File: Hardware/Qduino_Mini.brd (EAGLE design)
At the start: 38.1 x 25.4 mm, 45 parts, among them Q1 PFET, U1 ATMEGA32U41:1-LESS_PASTE, U2 MCP73831, U3 MAX17048, U4 TPS78233, U5 MIGHTYQ-L-SILK, U6 MIGHTYQ-S-SILK, U7 DNP, Y1 8MHZ

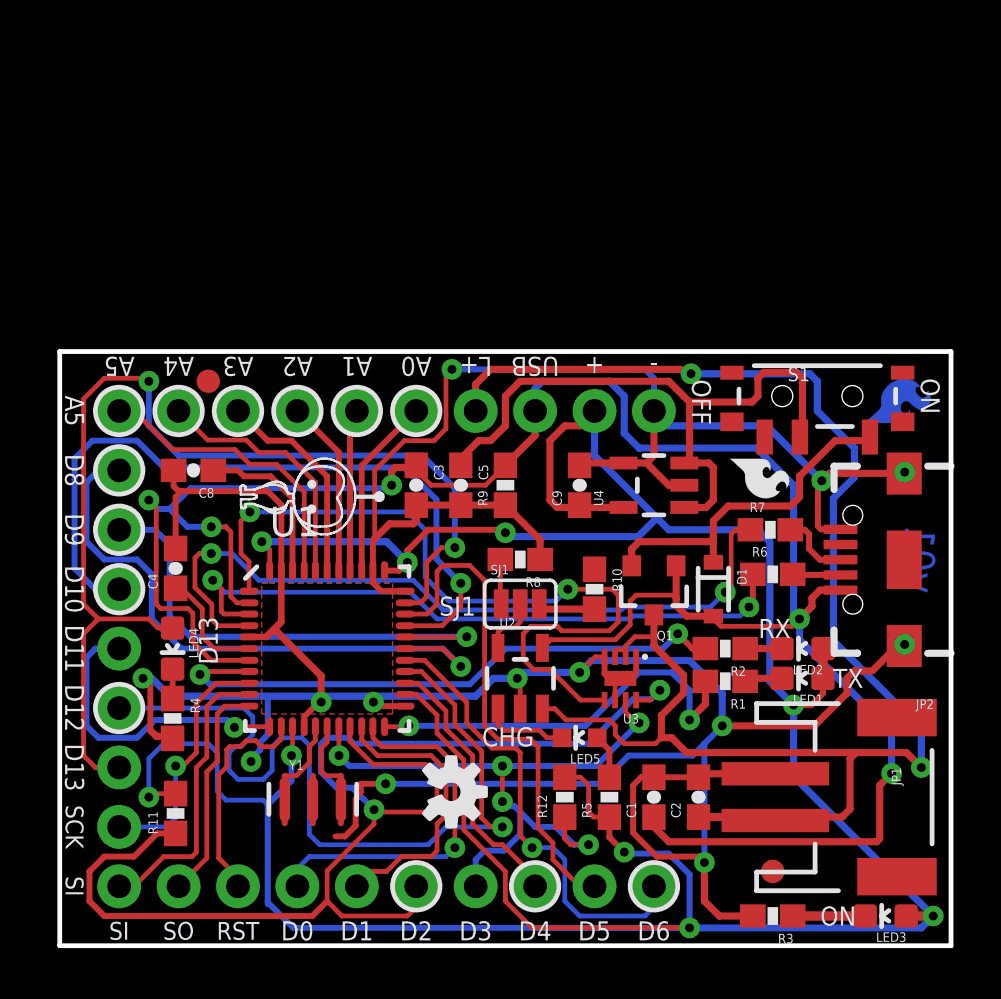
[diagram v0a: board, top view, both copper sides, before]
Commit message: Complete rework
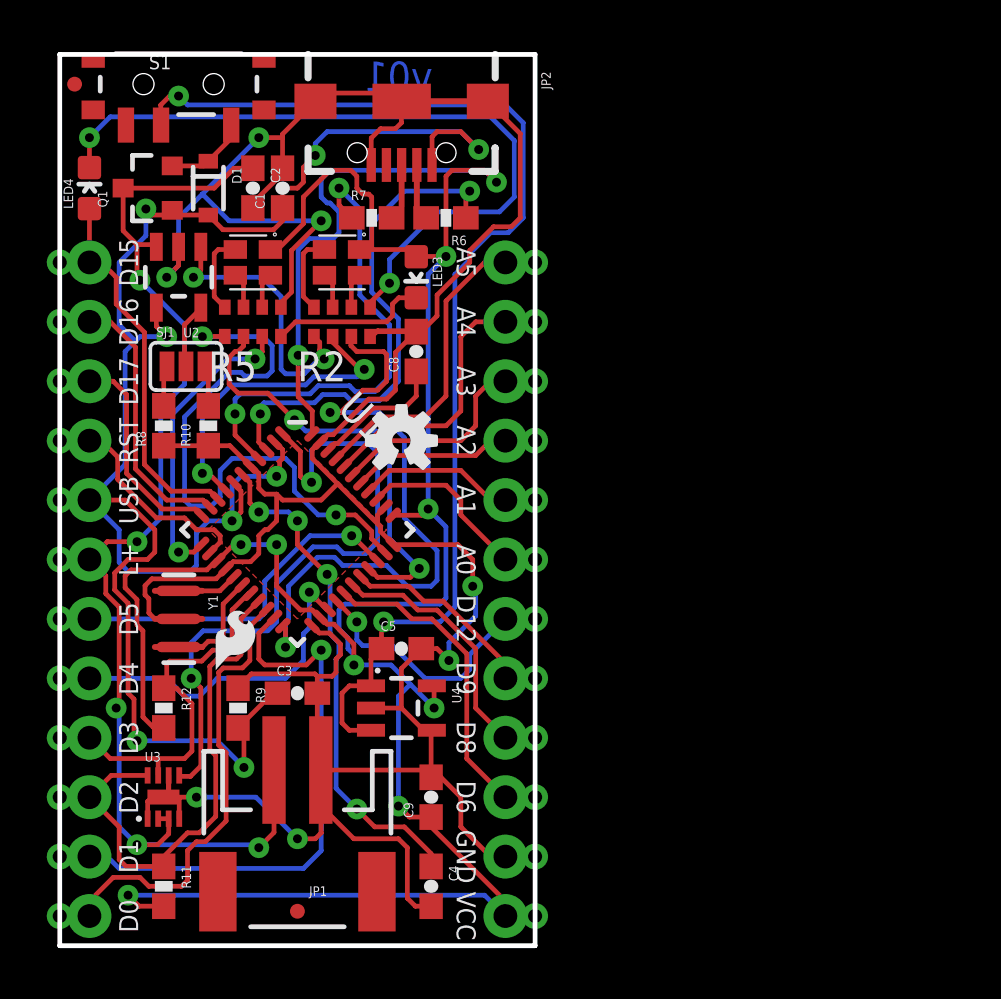
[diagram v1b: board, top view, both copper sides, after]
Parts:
- removed FID5, FID6: FIDUCIAL1X2, SparkFun-Aesthetics:FIDUCIAL-1X2
- removed LED5: CRG / RED, SparkFun:LED-0603
- removed R1, R3, R4: 330, SparkFun-Resistors:0603-RES
- removed U$6: (no value), SparkFun-Aesthetics:SFE-LOGO-FLAME-COPPER
- removed U6: MIGHTYQ-S-SILK, SparkFun-Aesthetics:LOGO-SMALL-SILK
- removed U7: DNP, SparkFun-Aesthetics:QDUINO_MINI_V15
- added FID1, FID2: FIDUCIALUFIDUCIAL, SparkFun-Aesthetics:MICRO-FIDUCIAL
- added JP3, JP4: (no value), SparkFun-Connectors:1X12
- added LOGO3: SFE_LOGO_FLAME.1_INCH, SparkFun-Aesthetics:SFE_LOGO_FLAME_.1@1
- D1: value BAS16JTR -> 250mA/100V
- JP2: value USB_MICROB_PLUGCONN-11752 -> (none)
- LED1: value TX / YLW -> (none); device SparkFun-LED:LED-0603 -> Spark:PLCC4-2MM-RGB
- LED2: value RX / GRN -> (none); device SparkFun-LED:LED-0603 -> Spark:PLCC4-2MM-RGB
- R2, R5: device SparkFun-Resistors:0603-RES -> SparkFun-Passives:0603-ARV
- U4: value TPS78233 -> AP2112K-3.3TRG-1
- moved LED3 33.9 mm to (15.2, 28.6), turned to 180 degrees
- moved C2 32.3 mm to (8.26, 32.4), turned to 270 degrees
- moved C1 30.5 mm to (9.53, 32.4)
- moved S1 30.4 mm to (5.08, 36.8)
- moved JP2 29.1 mm to (14.6, 36.1), turned to 270 degrees
- moved LED2 28.7 mm to (8.26, 29.2)
- moved LOGO2 28.4 mm to (3.17, 34.3), flipped to the bottom, turned to 0 degrees
- moved D1 27.6 mm to (6.35, 32.4)
- moved Q1 27.6 mm to (3.81, 32.4), turned to 90 degrees
- moved LED1 26.5 mm to (12.1, 29.2)
- moved R5 25.4 mm to (8.26, 26.7), turned to 0 degrees
- moved JP1 24.3 mm to (10.2, 3.81), turned to 180 degrees
- moved U2 22.5 mm to (5.08, 28.6), turned to 180 degrees
- moved R7 21.6 mm to (13.3, 31.1)
- moved R2 21.5 mm to (12.1, 26.7), turned to 0 degrees
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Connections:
- removed net N$12: LED3.C, R3.1
- new net N$32: LED2.BLUE, R5.6
- new net N$34: LED1.GREEN, R2.7
- new net N$35: LED2.RED, R5.8
- new net N$37: LED2.GREEN, R5.7
- net A0: now also JP3.7; no longer U7.A0
- net A1: now also JP3.8; no longer U7.A1
- net A2: now also JP3.9; no longer U7.A2
- net A3: now also JP3.10; no longer U7.A3
- net A4: now also JP3.11; no longer U7.A4
- net A5: now also JP3.12; no longer U7.A5
- net D10: now also R5.2; no longer U7.D10
- net D11: now also R5.3; no longer U7.D11
- net D12: now also JP3.6; no longer U7.D12
- net D13: now also R5.1; no longer LED4.A, U7.D31
- net D4: now also JP4.5; no longer U7.D4
- net D5: now also JP4.6; no longer U7.D5
- net D6: now also JP3.3; no longer U7.D6
- net D8: now also JP3.4; no longer U7.D8
- net D9: now also JP3.5; no longer U7.D9
- net GND: now also JP3.2, R2.4, R5.5; no longer R3.2, R4.2, U7.GND
- net LIPO: now also JP4.7; no longer U7.LIPO
- net MISO: now also JP4.10; no longer U7.MISO
- net MOSI: now also JP4.11; no longer U7.MOSI
- net N$1: now also LED1.RED, R2.8; no longer LED1.C, R1.1
- net N$2: now also LED1.BLUE, R2.6; no longer LED2.C, R2.1
- net N$4: now also LED3.C, R5.4; no longer LED5.A, R5.2
- net N$5: now also R2.5; no longer R4.1
- net RST: now also JP4.9; no longer U7.RST
- net RX: now also JP4.1; no longer U7.TX
- net RXLED: now also R2.3, U1.22; no longer R2.2, U1.8
- net SCK: now also JP4.12, LED4.A; no longer U7.SCK
- net SCL: now also JP4.4; no longer U7.D3
- net SDA: now also JP4.3; no longer U7.D2
- net STAT: now also R2.1; no longer LED5.C
- net TX: now also JP4.2; no longer U7.RX
- net TXLED: now also R2.2, U1.8; no longer R1.2, U1.22
- net VBUS: now also JP4.8; no longer U7.VUSB
- net VCC: now also JP3.1, LED1.CA, LED2.CA; no longer LED1.A, LED2.A, R5.1, U7.VCC
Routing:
- net SDA: track 56.3 -> 23.4 mm, vias 2 -> 1
- net N$5: track 1.26 -> 31.5 mm, vias 0 -> 2
- net D12: track 35.4 -> 11.7 mm, vias 1 -> 2
- net LIPO: track 74.6 -> 52.1 mm, vias 2 -> 6
- net VINPUT: track 27.8 -> 49.6 mm, vias 0 -> 2
- net D13: track 46.6 -> 26.1 mm
- net VCC: track 142.9 -> 122.8 mm, vias 9 -> 11
- net VBUS: track 98.6 -> 80.2 mm, vias 5 -> 9
- net GND: track 168.4 -> 151.1 mm, vias 13 -> 8
- net UCAP: track 4.91 -> 21.7 mm, vias 0 -> 4
- net D8: track 26.2 -> 12.0 mm
- net D10: track 31.5 -> 18.7 mm, vias 1 -> 2
- net D+: track 32.2 -> 20.6 mm
- net D9: track 21.2 -> 9.62 mm
- net SCL: track 28.8 -> 17.2 mm, vias 5 -> 1
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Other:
- board size 38.1 x 25.4 mm -> 20.3 x 38.1 mm
- board text added: "A0"
- board text added: "A1"
- board text added: "A2"
- board text added: "A3"
- board text added: "A4"
- board text added: "A5"
- board text added: "D0"
- board text added: "D1"
- board text added: "D12"
- board text added: "D15"
- board text added: "D16"
- board text added: "D17"
- board text added: "D2"
- board text added: "D3"
- board text added: "D4"
- board text added: "D5"
- board text added: "D6"
- board text added: "D8"
- board text added: "D9"
- board text added: "GND"
- board text added: "L+"
- board text added: "LIPO"
- board text added: "MISO"
- board text added: "MOSI"
- board text added: "RST"
- board text added: "SCK"
- board text added: "SCL"
- board text added: "SDA"
- board text added: "USB"
- board text added: "VCC"
- board text removed: "All units in inches"
- board text removed: "CHG"
- board text removed: "D13"
- board text removed: "OFF"
- board text removed: "ON"
- board text removed: "SJ1"
